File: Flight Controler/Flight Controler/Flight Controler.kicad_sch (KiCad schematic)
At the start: 15 parts, among them U1 STM32F415RGTx, U2 MPU-6050, U3 BMI160, U4 BMP280

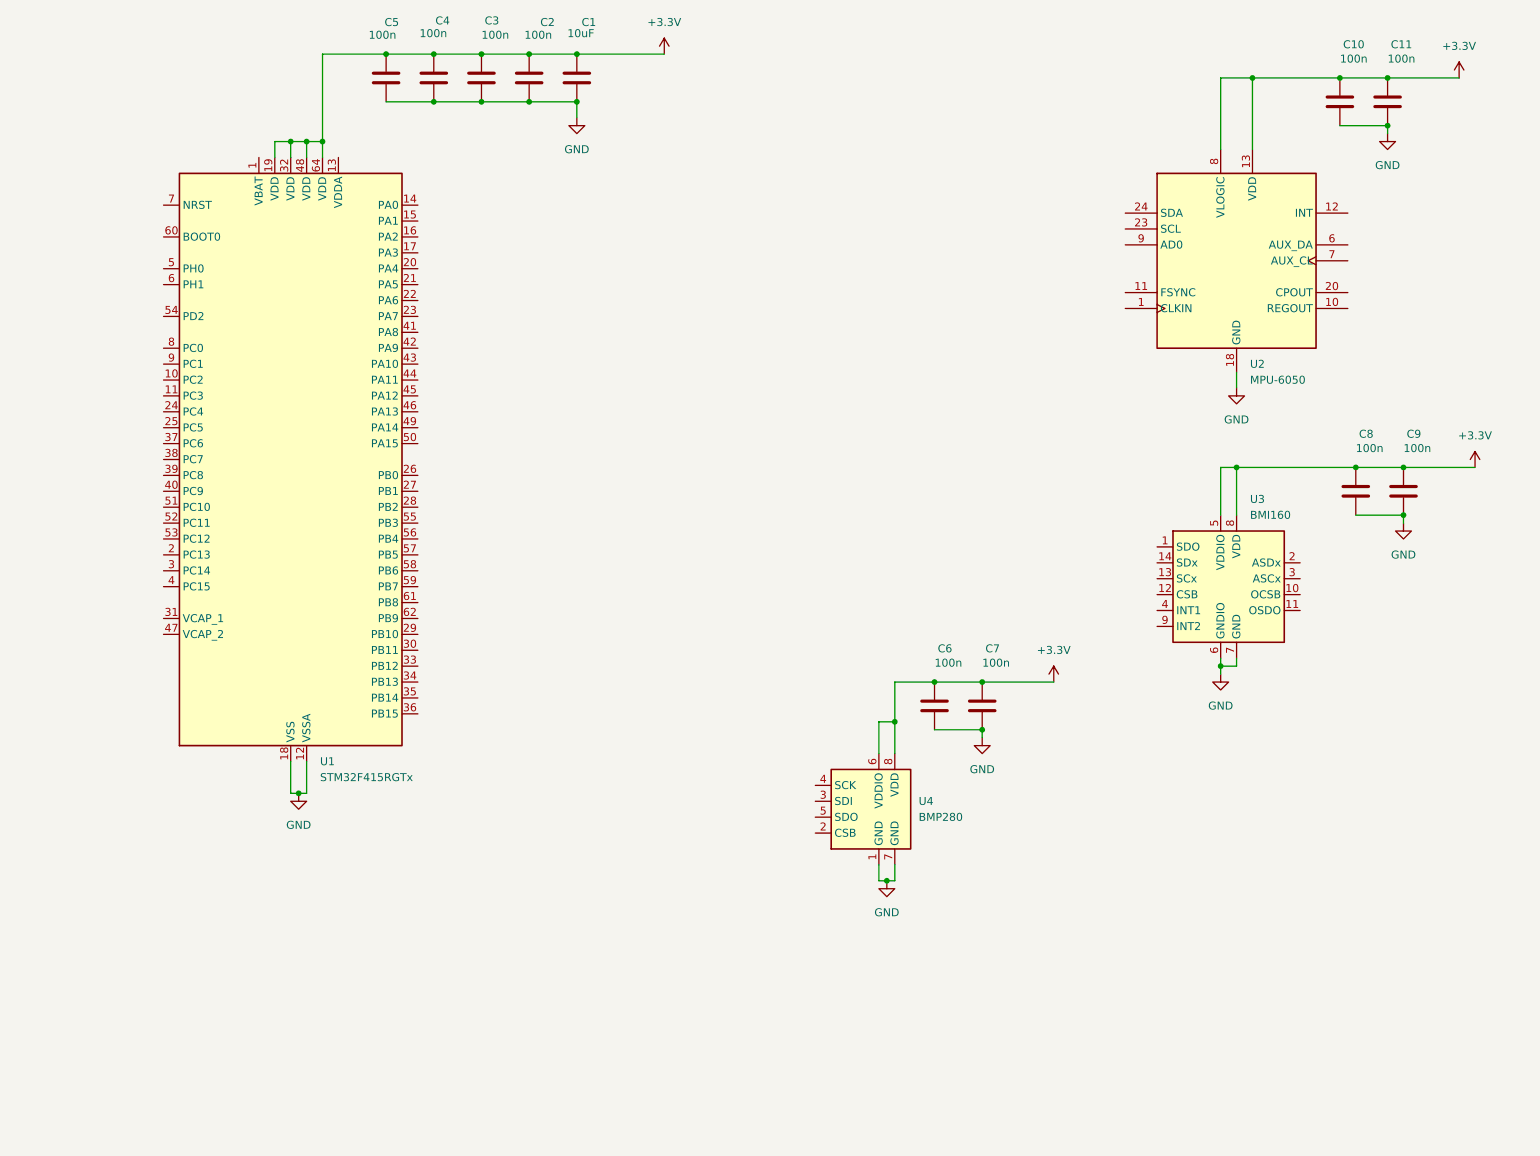
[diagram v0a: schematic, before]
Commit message: klein update
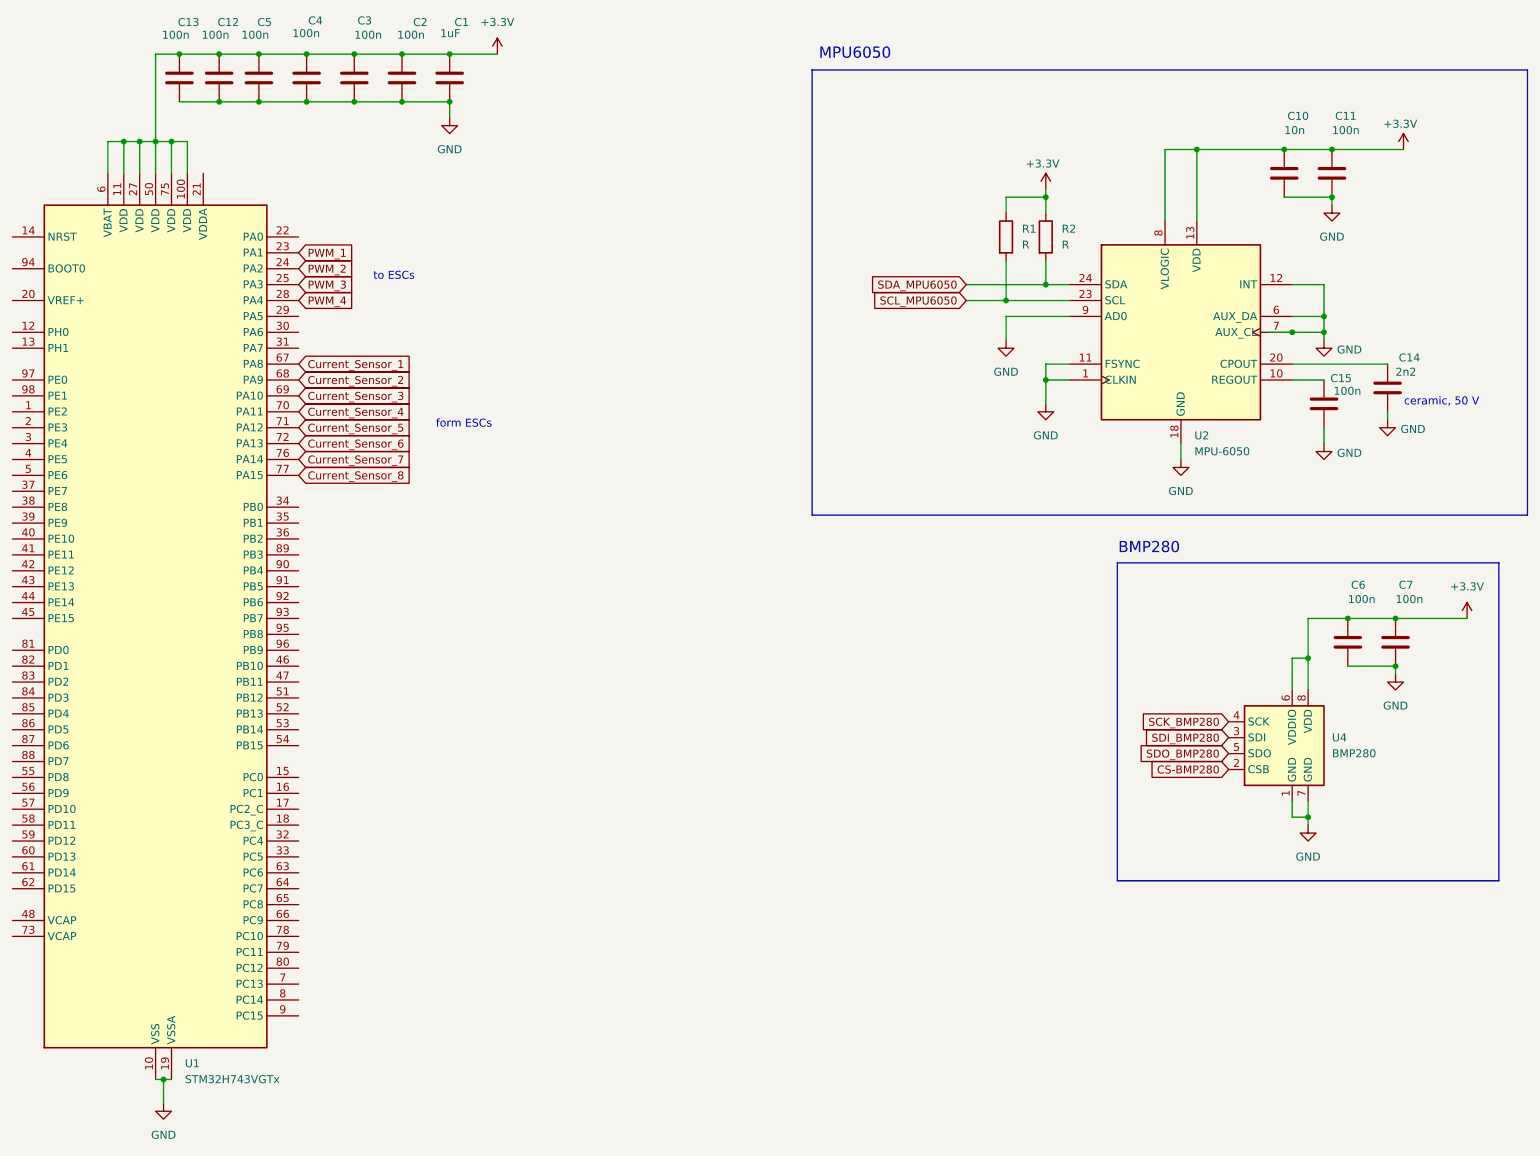
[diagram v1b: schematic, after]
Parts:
- removed C8, C9: 100n, symbol Device:C
- removed U1: STM32F415RGTx, Package_QFP:LQFP-64_10x10mm_P0.5mm, symbol MCU_ST_STM32F4:STM32F415RGTx
- removed U3: BMI160, Package_LGA:Bosch_LGA-14_3x2.5mm_P0.5mm, symbol Sensor_Motion:BMI160
- added C12, C13, C15: 100n, symbol Device:C
- added C14: 2n2, symbol Device:C
- added R1, R2: R, symbol Device:R
- added U1: STM32H743VGTx, Package_QFP:LQFP-100_14x14mm_P0.5mm, symbol MCU_ST_STM32H7:STM32H743VGTx
- C1: value 10uF -> 1uF
- C10: value 100n -> 10n
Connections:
- net +3.3V: now also C12.1, C13.1, R1.1, R2.1, U1.100 (VDD), U1.11 (VDD), U1.27 (VDD), U1.50 (VDD), U1.6 (VBAT), U1.75 (VDD)
- net GND: now also U2.1 (CLKIN), U2.11 (FSYNC), U2.12 (INT), U2.6 (AUX_DA), U2.7 (AUX_CL), U2.9 (AD0), C12.2, C13.2, C14.2, C15.2, U1.10 (VSS), U1.19 (VSSA), U1.26 (VSS), U1.49 (VSS), U1.74 (VSS), U1.99 (VSS)
- net CS-BMP280: now reaches U4.2 (CSB)
- net SDI_BMP280: now reaches U4.3 (SDI)
- net SCK_BMP280: now reaches U4.4 (SCK)
- net SDO_BMP280: now reaches U4.5 (SDO)
- net at U2.10 (REGOUT): now also C15.1
- net at U2.20 (CPOUT): now also C14.1
- net SCL_MPU6050: now reaches U2.23 (SCL)
- net SCL_MPU6050: now also R1.2
- net SDA_MPU6050: now reaches U2.24 (SDA)
- net SDA_MPU6050: now also R2.2
- new net Current_Sensor_1: U1.67 (PA8)
- new net Current_Sensor_2: U1.68 (PA9)
- new net Current_Sensor_3: U1.69 (PA10)
- new net Current_Sensor_4: U1.70 (PA11)
- new net Current_Sensor_5: U1.71 (PA12)
- new net Current_Sensor_6: U1.72 (PA13)
- new net Current_Sensor_7: U1.76 (PA14)
- new net Current_Sensor_8: U1.77 (PA15)
- new net PWM_1: U1.23 (PA1)
- new net PWM_2: U1.24 (PA2)
- new net PWM_3: U1.25 (PA3)
- new net PWM_4: U1.28 (PA4)
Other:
- note added: "BMP280"
- note added: "MPU6050"
- note added: "ceramic, 50 V"
- note added: "form ESCs"
- note added: "to ESCs"
- moved on the sheet: C1, C10, C11, C2, C3, C4, C5, C6, C7, U2, U4

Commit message: update
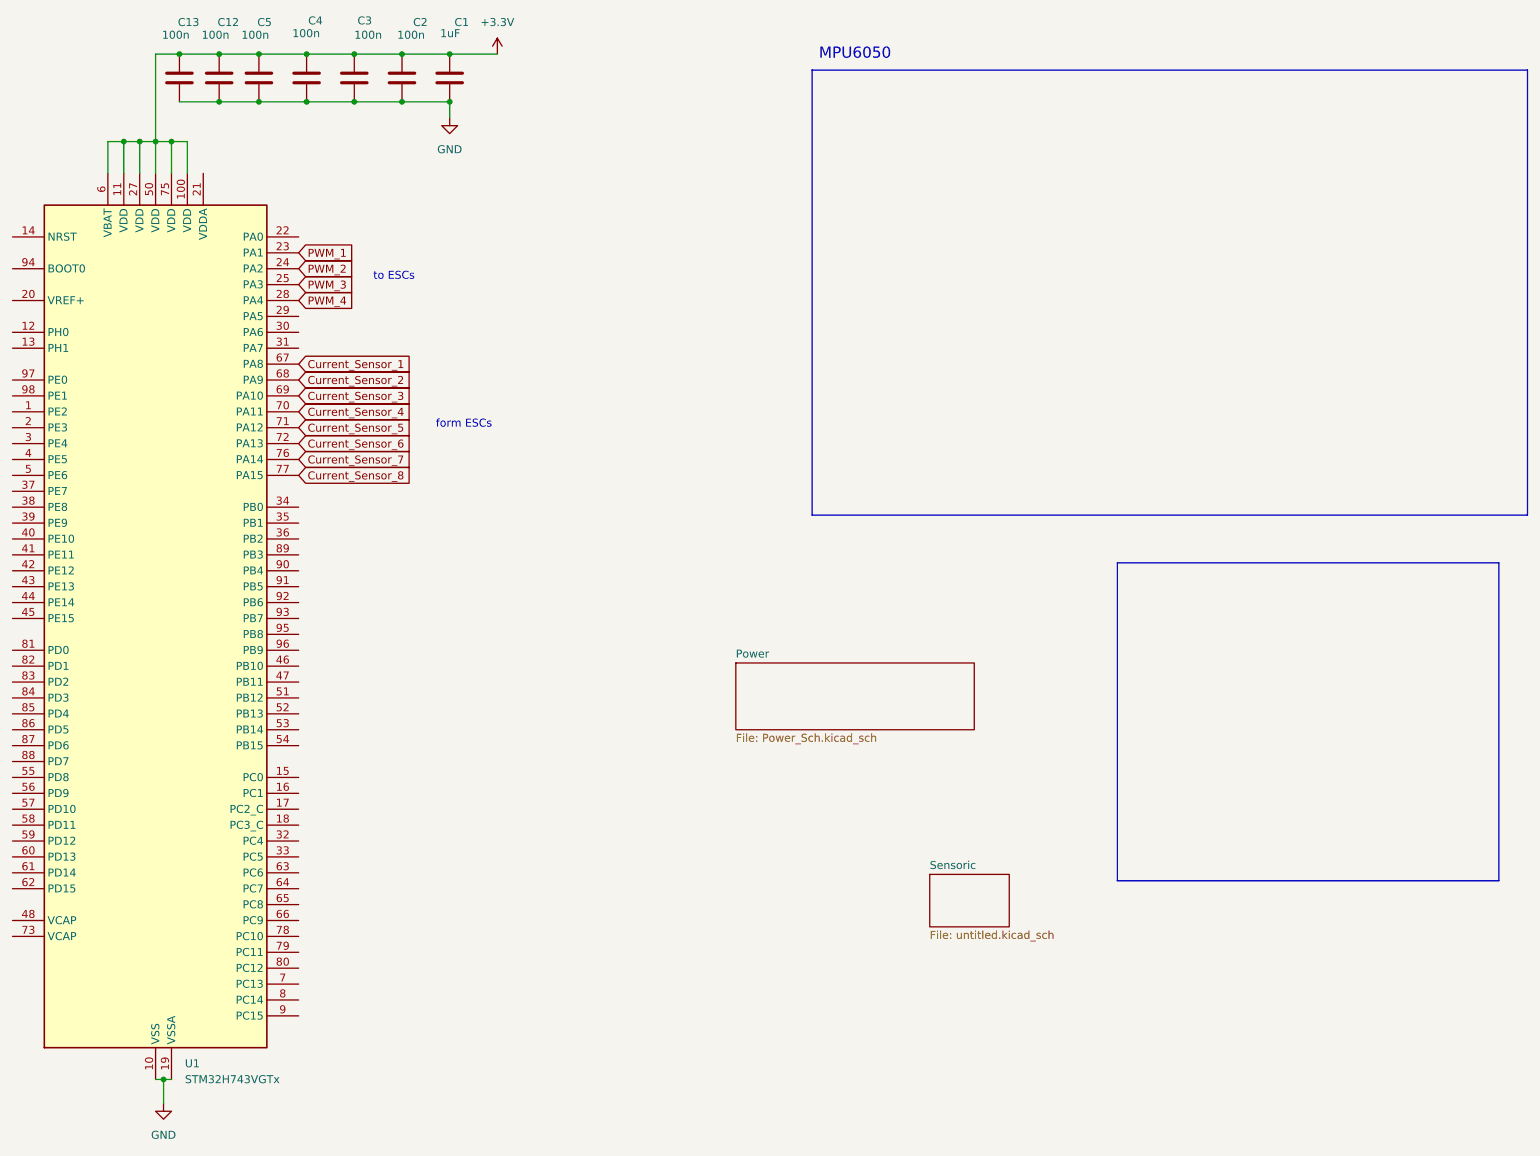
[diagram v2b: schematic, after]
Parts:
- removed C10: 10n, symbol Device:C
- removed C11, C15, C6, C7: 100n, symbol Device:C
- removed C14: 2n2, symbol Device:C
- removed R1, R2: R, symbol Device:R
- removed U2: MPU-6050, Sensor_Motion:InvenSense_QFN-24_4x4mm_P0.5mm, symbol Sensor_Motion:MPU-6050
- removed U4: BMP280, Package_LGA:Bosch_LGA-8_2x2.5mm_P0.65mm_ClockwisePinNumbering, symbol Sensor_Pressure:BMP280
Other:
- added sheet Power (Power_Sch.kicad_sch)
- added sheet Sensoric (untitled.kicad_sch)
- note removed: "BMP280"
- note removed: "ceramic, 50 V"
